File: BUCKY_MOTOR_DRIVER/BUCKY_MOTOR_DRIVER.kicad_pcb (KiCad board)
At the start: 2 copper layers, 26 x 22.6 mm, 8 parts, among them J1 P_INPUTS, J2 INPUTS, J3 OUT, U1 IFX9201SG

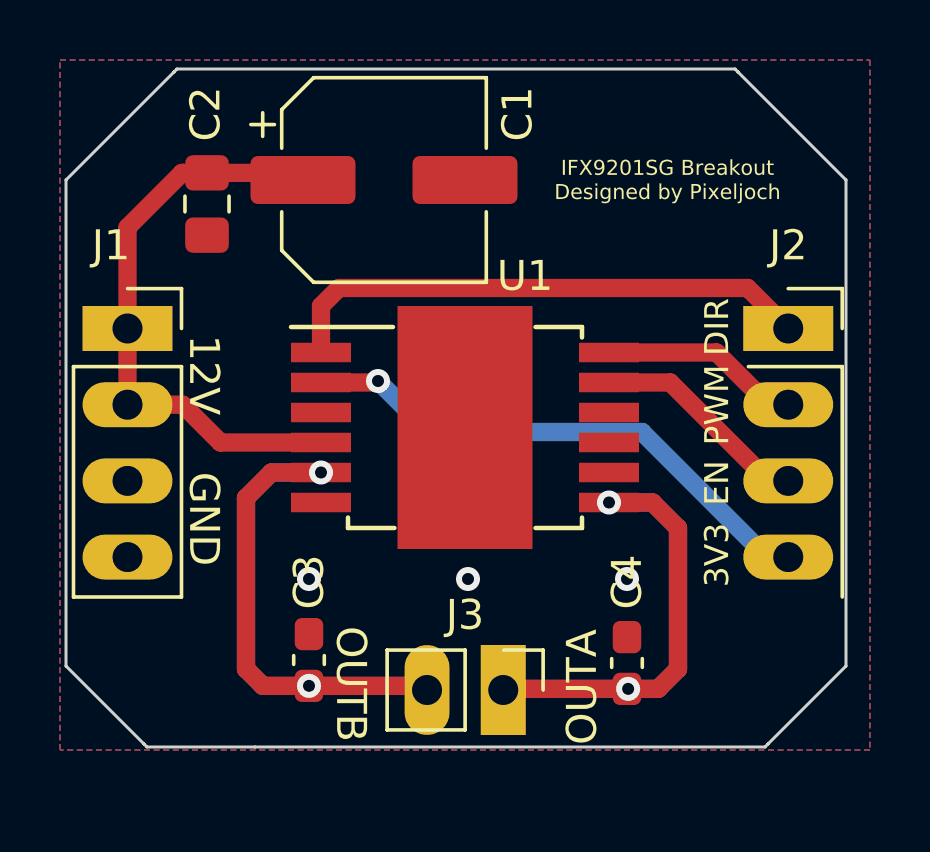
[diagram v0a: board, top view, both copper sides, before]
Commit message: Finished PCBS
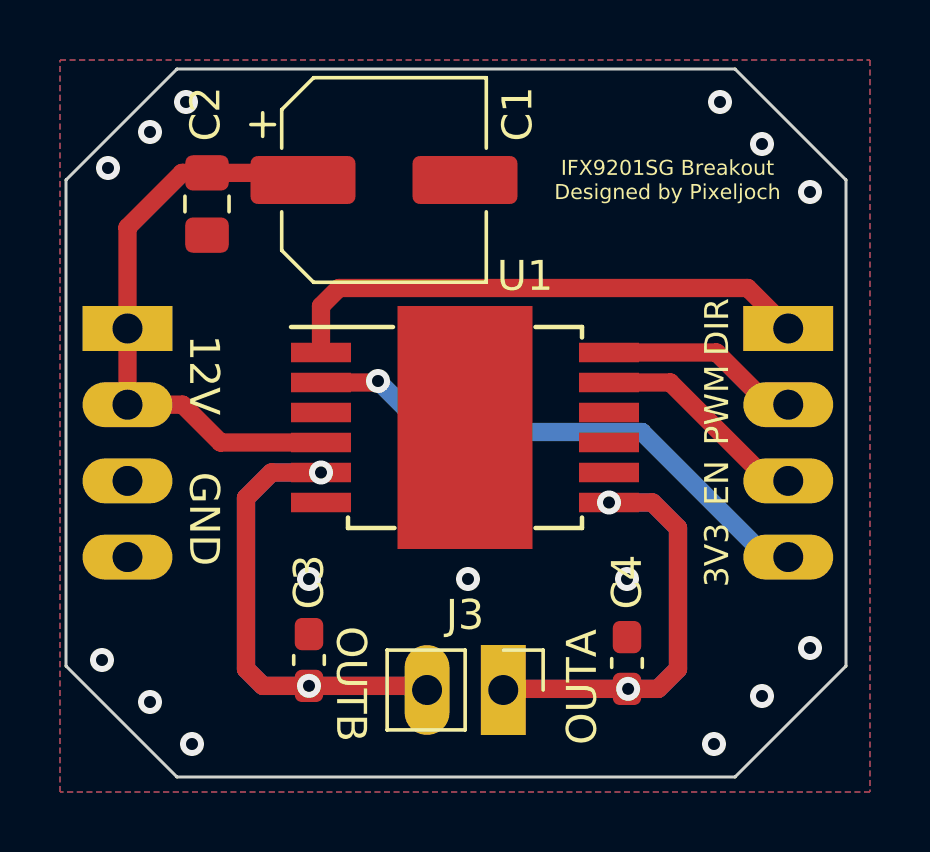
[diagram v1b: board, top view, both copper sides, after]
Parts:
- J1, J2: moved to B.Cu
- turned J1 to 180 degrees
- turned J2 to 180 degrees
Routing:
- net GND: vias 3 -> 15
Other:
- board size 26 x 22.6 mm -> 26 x 23.6 mm
